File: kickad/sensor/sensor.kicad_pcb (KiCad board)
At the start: 4 copper layers, 34.9 x 19 mm, 13 parts, among them J3 trackball, U1 MCP1700x-180xxTT, U2 PMW3610

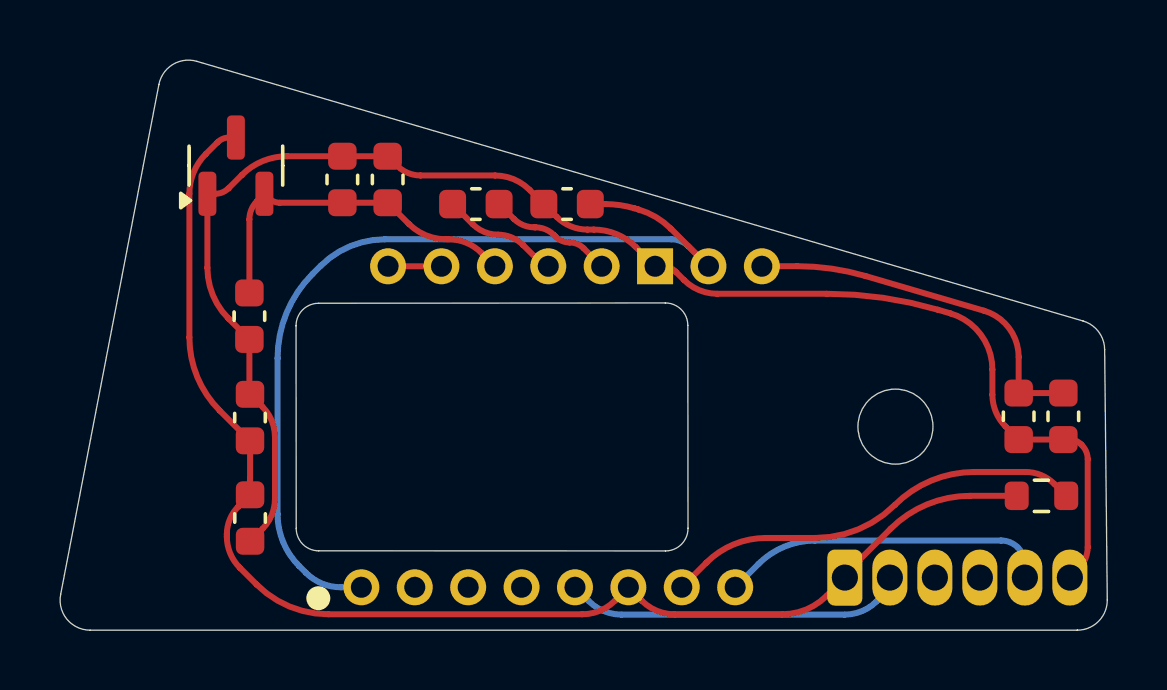
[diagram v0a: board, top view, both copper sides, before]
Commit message: Releasing all the gerbers
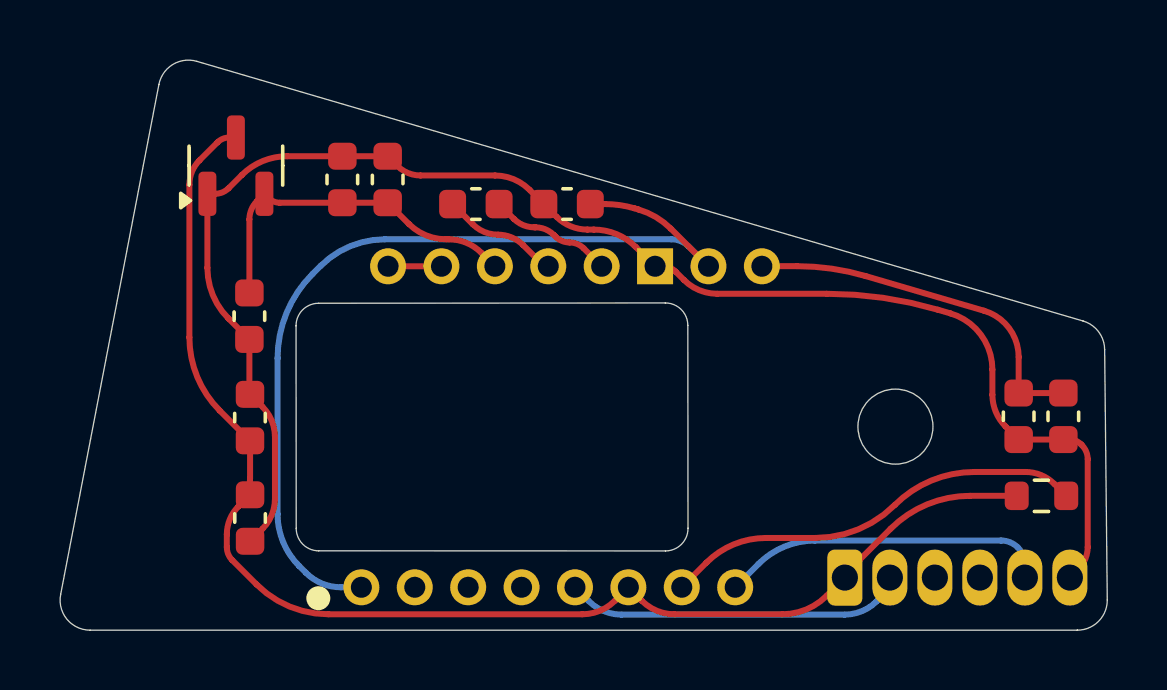
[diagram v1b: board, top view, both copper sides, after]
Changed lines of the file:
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@@
 	)
 	(segment
-		(start 136.022059 94.496042)
+		(start 136.022155 94.496138)
 		(end 135.964009 94.437992)
 		(width 0.2)
@@
 	)
 	(arc
-		(start 136.022059 94.496042)
-		(mid 136.237441 94.639956)
+		(start 136.022155 94.496138)
+		(mid 136.237431 94.639981)
 		(end 136.491501 94.690492)
 		(width 0.2)
@@
 	(segment
 		(start 125.065 104.423007)
-		(end 125.065 104.486848)
+		(end 125.065 104.844371)
 		(width 0.2)
 		(layer "F.Cu")
@@
 	(segment
 		(start 126.057591 106.091287)
-		(end 125.497641 105.531337)
-		(width 0.2)
-		(layer "F.Cu")
-		(net 5)
-	)
-	(segment
-		(start 124.365891 91.740586)
+		(end 125.244834 105.27853)
+		(width 0.2)
+		(layer "F.Cu")
+		(net 5)
+	)
+	(segment
+		(start 124.156395 91.950081)
 		(end 124.754187 91.352291)
 		(width 0.2)
@@
 	)
 	(segment
-		(start 123.817418 93.06472)
+		(start 123.817418 92.768443)
 		(end 123.817418 97.853757)
 		(width 0.2)
@@
 	)
 	(arc
-		(start 125.065 104.486848)
-		(mid 125.177439 105.052121)
-		(end 125.497641 105.531337)
+		(start 125.065 104.844371)
+		(mid 125.111737 105.079336)
+		(end 125.244834 105.27853)
 		(width 0.2)
 		(layer "F.Cu")
@@
 	)
 	(arc
-		(start 124.365891 91.740586)
-		(mid 123.959961 92.348104)
-		(end 123.817418 93.06472)
-		(width 0.2)
-		(layer "F.Cu")
+		(start 124.156395 91.950081)
+		(mid 123.905515 92.325549)
+		(end 123.817418 92.768443)
+		(width 0.2)
+		(layer "F.Cu")
